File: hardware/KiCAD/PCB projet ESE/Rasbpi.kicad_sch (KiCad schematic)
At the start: 4 parts, among them J17 Conn_01x02

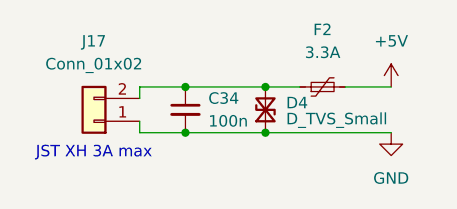
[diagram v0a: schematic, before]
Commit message: v1 PCB
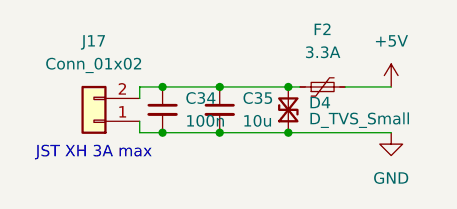
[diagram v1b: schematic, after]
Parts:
- added C35: 10u, Capacitor_SMD:C_0402_1005Metric, symbol Device:C_Small
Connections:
- net GND: now also C35.2
- net at C34.1, D4.2 (A2), F2.1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: now also C35.1
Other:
- moved on the sheet: C34, D4
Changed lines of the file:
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@@
 	)
 	(junction
-		(at 238.76 57.15)
+		(at 233.68 62.23)
 		(diameter 0)
 		(color 0 0 0 0)
 	)
 	(junction
-		(at 229.87 57.15)
+		(at 233.68 57.15)
 		(diameter 0)
 		(color 0 0 0 0)
 	)
 	(junction
-		(at 238.76 62.23)
+		(at 241.3 62.23)
 		(diameter 0)
 		(color 0 0 0 0)
 	)
 	(junction
-		(at 229.87 62.23)
+		(at 227.33 57.15)
 		(diameter 0)
 		(color 0 0 0 0)
 	)
+	(junction
+		(at 227.33 62.23)
+		(diameter 0)
+		(color 0 0 0 0)
+	)
+	(junction
+		(at 241.3 57.15)
+		(diameter 0)
+		(color 0 0 0 0)
+	)
 	(wire
 		(pts
@@
 	(wire
 		(pts
-			(xy 229.87 62.23) (xy 238.76 62.23)
-		)
-		(stroke
-			(width 0)
-			(type default)
-		)
-	)
-	(wire
-		(pts
-			(xy 238.76 57.15) (xy 242.57 57.15)
-		)
-		(stroke
-			(width 0)
-			(type default)
-		)
-	)
-	(wire
-		(pts
-			(xy 229.87 57.15) (xy 224.79 57.15)
+			(xy 227.33 62.23) (xy 233.68 62.23)
+		)
+		(stroke
+			(width 0)
+			(type default)
+		)
+	)
+	(wire
+		(pts
+			(xy 241.3 62.23) (xy 252.73 62.23)
+		)
+		(stroke
+			(width 0)
+			(type default)
+		)
+	)
+	(wire
+		(pts
+			(xy 227.33 57.15) (xy 233.68 57.15)
 		)
 		(stroke
@@
 	(wire
 		(pts
-			(xy 238.76 62.23) (xy 252.73 62.23)
-		)
-		(stroke
-			(width 0)
-			(type default)
-		)
-	)
-	(wire
-		(pts
-			(xy 224.79 62.23) (xy 229.87 62.23)
+			(xy 233.68 62.23) (xy 241.3 62.23)
+		)
+		(stroke
+			(width 0)
+			(type default)
+		)
+	)
+	(wire
+		(pts
+			(xy 241.3 57.15) (xy 242.57 57.15)
+		)
+		(stroke
+			(width 0)
+			(type default)
+		)
+	)
+	(wire
+		(pts
+			(xy 224.79 62.23) (xy 227.33 62.23)
+		)
+		(stroke
+			(width 0)
+			(type default)
+		)
+	)
+	(wire
+		(pts
+			(xy 233.68 57.15) (xy 241.3 57.15)
+		)
+		(stroke
+			(width 0)
+			(type default)
+		)
+	)
+	(wire
+		(pts
+			(xy 227.33 57.15) (xy 224.79 57.15)
 		)
 		(stroke
@@
 		(pts
 			(xy 224.79 57.15) (xy 224.79 58.42)
-		)
-		(stroke
-			(width 0)
-			(type default)
-		)
-	)
-	(wire
-		(pts
-			(xy 229.87 57.15) (xy 238.76 57.15)
 		)
 		(stroke
@@
 	(symbol
 		(lib_id "Device:C_Small")
-		(at 229.87 59.69 0)
+		(at 233.68 59.69 0)
+		(unit 1)
+		(exclude_from_sim no)
+		(in_bom yes)
+		(on_board yes)
+		(dnp no)
+		(property "Reference" "C35"
+			(at 236.22 58.4262 0)
+			(effects
+				(font
+					(size 1.27 1.27)
+				)
+				(justify left)
+			)
+		)
+		(property "Value" "10u"
+			(at 236.22 60.96 0)
+			(effects
+				(font
+					(size 1.27 1.27)
+				)
+				(justify left)
+			)
+		)
+		(property "Footprint" "Capacitor_SMD:C_0402_1005Metric"
+			(at 233.68 59.69 0)
+			(effects
+				(font
+					(size 1.27 1.27)
+				)
+				(hide yes)
+			)
+		)
+		(property "Datasheet" "~"
+			(at 233.68 59.69 0)
+			(effects
+				(font
+					(size 1.27 1.27)
+				)
+				(hide yes)
+			)
+		)
+		(property "Description" "Unpolarized capacitor, small symbol"
+			(at 233.68 59.69 0)
+			(effects
+				(font
+					(size 1.27 1.27)
+				)
+				(hide yes)
+			)
+		)
+		(pin "1"
+		)
+		(pin "2"
+		)
+		(instances
+			(project "PCB projet ESE"
+				(path "/61bc2d2d-cd10-4636-b1b1-3d875f78e40b/7a080ce4-c82c-46c4-8a5a-914178d680a1"
+					(reference "C35")
+					(unit 1)
+				)
+			)
+		)
+	)
+	(symbol
+		(lib_id "Device:C_Small")
+		(at 227.33 59.69 0)
 		(unit 1)
 		(exclude_from_sim no)
@@
 		(dnp no)
 		(property "Reference" "C34"
-			(at 232.41 58.4262 0)
+			(at 229.87 58.4262 0)
 			(effects
 				(font
@@
 		)
 		(property "Value" "100n"
-			(at 232.41 60.96 0)
+			(at 229.87 60.96 0)
 			(effects
 				(font
@@
 		)
 		(property "Footprint" "Capacitor_SMD:C_0402_1005Metric"
-			(at 229.87 59.69 0)
+			(at 227.33 59.69 0)
 			(effects
 				(font
@@
 		)
 		(property "Datasheet" "~"
-			(at 229.87 59.69 0)
+			(at 227.33 59.69 0)
 			(effects
 				(font
@@
 		)
 		(property "Description" "Unpolarized capacitor, small symbol"
-			(at 229.87 59.69 0)
+			(at 227.33 59.69 0)
 			(effects
 				(font
@@
 	(symbol
 		(lib_id "Device:D_TVS_Small")
-		(at 238.76 59.69 90)
+		(at 241.3 59.69 90)
 		(unit 1)
 		(exclude_from_sim no)
@@
 		(dnp no)
 		(property "Reference" "D4"
-			(at 241.046 58.928 90)
+			(at 243.586 58.928 90)
 			(effects
 				(font
@@
 		)
 		(property "Value" "D_TVS_Small"
-			(at 241.046 60.706 90)
+			(at 243.586 60.706 90)
 			(effects
 				(font
@@
 		)
 		(property "Footprint" "Diode_SMD:D_SOD-523"
-			(at 238.76 59.69 0)
+			(at 241.3 59.69 0)
 			(effects
 				(font
@@
 		)
 		(property "Datasheet" "~"
-			(at 238.76 59.69 0)
+			(at 241.3 59.69 0)
 			(effects
 				(font
@@
 		)
 		(property "Description" "Bidirectional transient-voltage-suppression diode, small symbol"
-			(at 238.76 59.69 0)
-			(effects
-				(font
+			(at 241.3 59.69 0)
+			(effects
+				(font
